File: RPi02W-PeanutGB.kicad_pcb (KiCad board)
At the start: 4 copper layers, 100 x 100 mm, 62 parts, among them J1 Raspberry_Pi_2_3, J3 AudioJack3_SwitchTR, J4 Conn_01x50, J5 Conn_02x10_Odd_Even, J6 Conn_02x10_Odd_Even, J7 Conn_02x10_Odd_Even, J8 Conn_02x10_Odd_Even, J9 USB_C_Receptacle, SW1 SW_SPDT_MSM, SW10 SW_Push, SW11 SW_Push, SW12 SW_Push, SW13 SW_Push, SW14 SW_Push, SW2 SW_Push, SW3 SW_Push, SW4 SW_Push, SW5 SW_Push, SW6 SW_Push, SW7 SW_Push, SW8 SW_Push, SW9 SW_Push, U1 MCP73831-2-OT, U3 LM4861MX

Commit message: Add files via upload
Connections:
- J1 pad 10: EXT-RXD -> unconnected-(J1-GPIO15/RXD-Pad10)
- J1 pad 3: EXT-SDA -> unconnected-(J1-SDA/GPIO2-Pad3)
- J1 pad 5: EXT-SCL -> unconnected-(J1-SCL/GPIO3-Pad5)
- J1 pad 8: EXT-TXD -> unconnected-(J1-GPIO14/TXD-Pad8)
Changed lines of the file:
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@@
   (net 12 "Net-(D1-K)")
   (net 13 "POWER")
-  (net 14 "EXT-SDA")
-  (net 15 "EXT-SCL")
+  (net 14 "unconnected-(J1-SDA{slash}GPIO2-Pad3)")
+  (net 15 "unconnected-(J1-SCL{slash}GPIO3-Pad5)")
   (net 16 "BUTTON-DU")
-  (net 17 "EXT-TXD")
-  (net 18 "EXT-RXD")
+  (net 17 "unconnected-(J1-GPIO14{slash}TXD-Pad8)")
+  (net 18 "unconnected-(J1-GPIO15{slash}RXD-Pad10)")
   (net 19 "BUTTON-START")
   (net 20 "BUTTON-RB")
@@
       (net 13 "POWER") (pinfunction "5V") (pintype "power_in"))
     (pad "3" thru_hole oval (at 0 -2.54 270) (size 1.7 1.7) (drill 1) (layers "*.Cu" "*.Mask")
-      (net 14 "EXT-SDA") (pinfunction "SDA/GPIO2") (pintype "bidirectional"))
+      (net 14 "unconnected-(J1-SDA{slash}GPIO2-Pad3)") (pinfunction "SDA/GPIO2") (pintype "bidirectional+no_connect"))
     (pad "4" thru_hole oval (at 2.54 -2.54 270) (size 1.7 1.7) (drill 1) (layers "*.Cu" "*.Mask")
       (net 13 "POWER") (pinfunction "5V") (pintype "passive"))
     (pad "5" thru_hole oval (at 0 -5.08 270) (size 1.7 1.7) (drill 1) (layers "*.Cu" "*.Mask")
-      (net 15 "EXT-SCL") (pinfunction "SCL/GPIO3") (pintype "bidirectional"))
+      (net 15 "unconnected-(J1-SCL{slash}GPIO3-Pad5)") (pinfunction "SCL/GPIO3") (pintype "bidirectional+no_connect"))
     (pad "6" thru_hole oval (at 2.54 -5.08 270) (size 1.7 1.7) (drill 1) (layers "*.Cu" "*.Mask")
       (net 2 "GND") (pinfunction "GND") (pintype "power_in"))
@@
       (net 16 "BUTTON-DU") (pinfunction "GCLK0/GPIO4") (pintype "bidirectional"))
     (pad "8" thru_hole oval (at 2.54 -7.62 270) (size 1.7 1.7) (drill 1) (layers "*.Cu" "*.Mask")
-      (net 17 "EXT-TXD") (pinfunction "GPIO14/TXD") (pintype "bidirectional"))
+      (net 17 "unconnected-(J1-GPIO14{slash}TXD-Pad8)") (pinfunction "GPIO14/TXD") (pintype "bidirectional+no_connect"))
     (pad "9" thru_hole oval (at 0 -10.16 270) (size 1.7 1.7) (drill 1) (layers "*.Cu" "*.Mask")
       (net 2 "GND") (pinfunction "GND") (pintype "passive"))
     (pad "10" thru_hole oval (at 2.54 -10.16 270) (size 1.7 1.7) (drill 1) (layers "*.Cu" "*.Mask")
-      (net 18 "EXT-RXD") (pinfunction "GPIO15/RXD") (pintype "bidirectional"))
+      (net 18 "unconnected-(J1-GPIO15{slash}RXD-Pad10)") (pinfunction "GPIO15/RXD") (pintype "bidirectional+no_connect"))
     (pad "11" thru_hole oval (at 0 -12.7 270) (size 1.7 1.7) (drill 1) (layers "*.Cu" "*.Mask")
       (net 19 "BUTTON-START") (pinfunction "GPIO17") (pintype "bidirectional"))

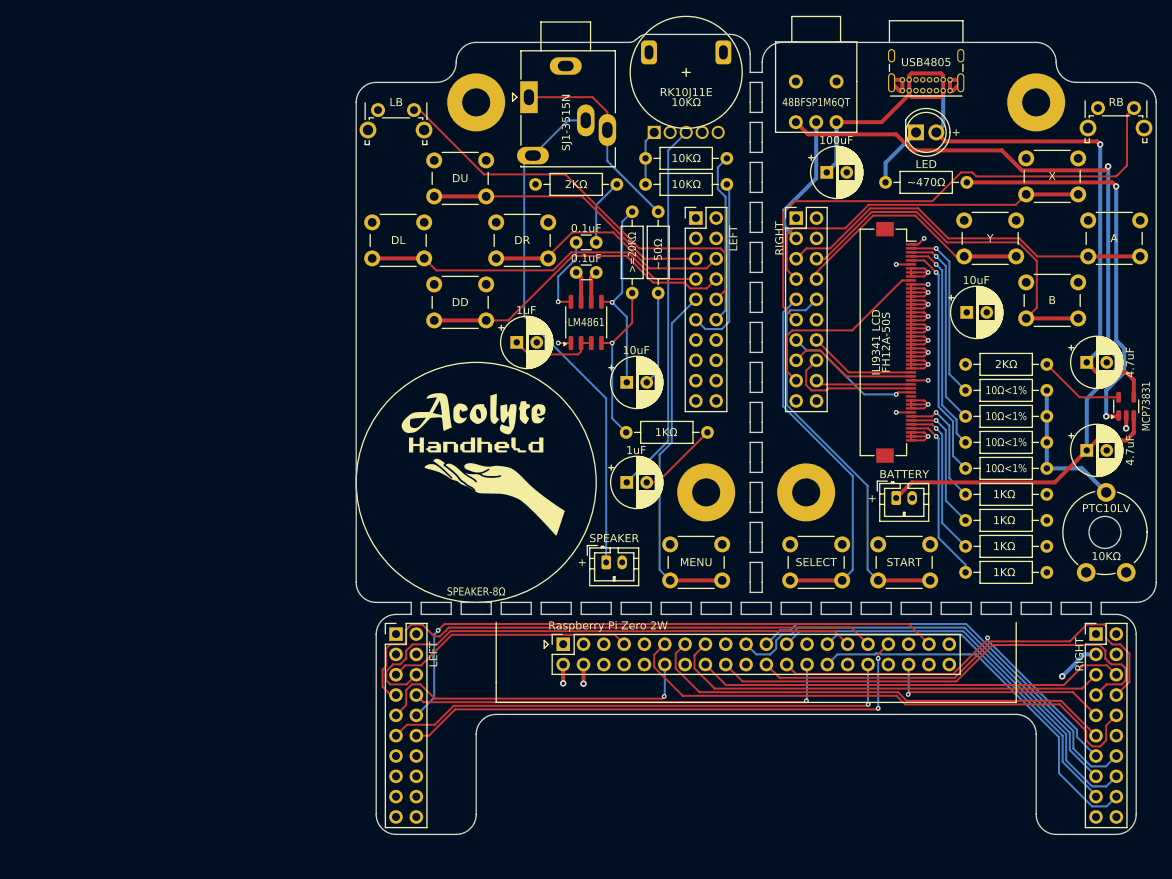
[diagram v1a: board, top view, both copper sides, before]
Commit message: Add files via upload
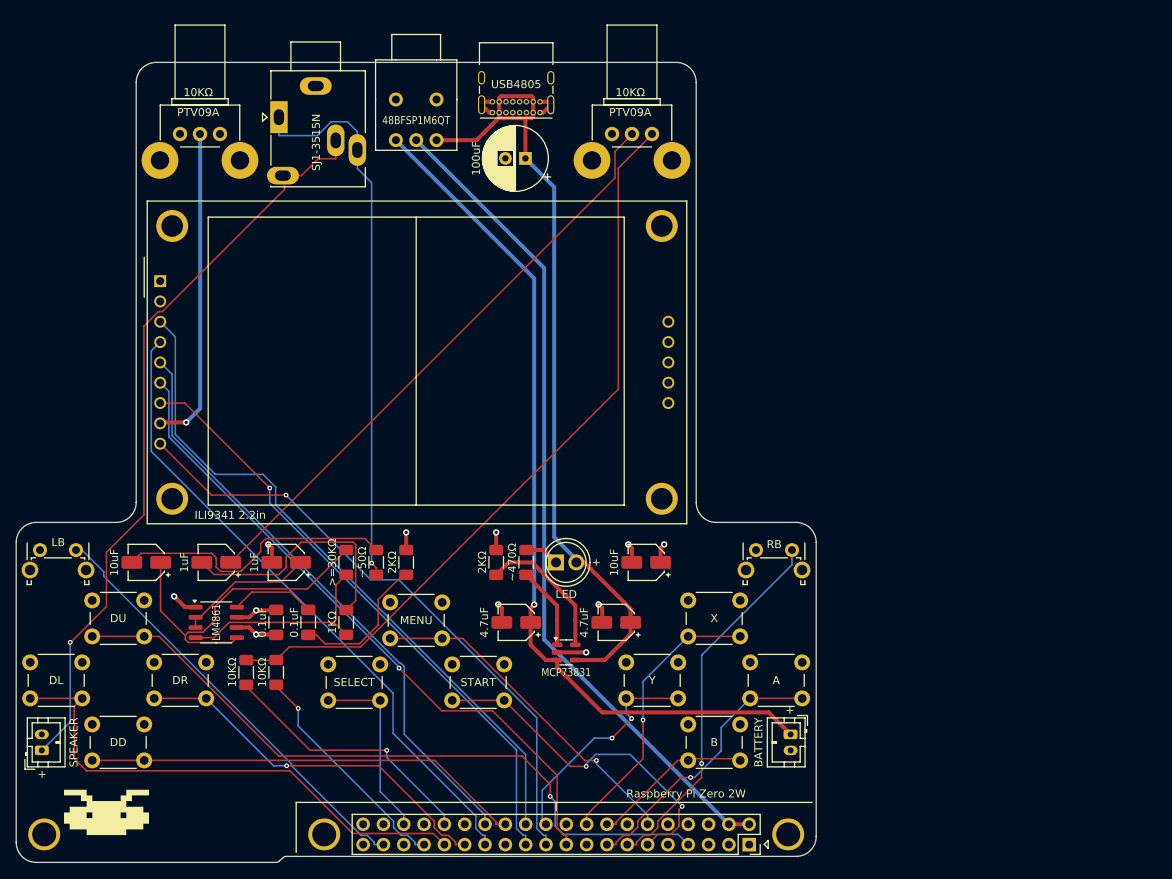
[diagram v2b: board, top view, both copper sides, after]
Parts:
- removed J4: Conn_01x50, Connector_FFC-FPC:Hirose_FH12-50S-0.5SH_1x50-1MP_P0.50mm_Horizontal
- removed J5, J6, J7, J8: Conn_02x10_Odd_Even, Connector_PinHeader_2.54mm:PinHeader_2x10_P2.54mm_Vertical
- removed R10, R11, R12, R13, R14, R15, R16, R9: R_US, Resistor_THT:R_Axial_DIN0207_L6.3mm_D2.5mm_P10.16mm_Horizontal
- removed RV1: R_Potentiometer_US, Potentiometer_THT:Potentiometer_Piher_PT-10-V10_Vertical_Hole
- removed TP4: TestPoint, RPi02W-PeanutGB:ScrewHole-4-40
- added G109: LOGO, RPi02W-PeanutGB:Alien, F.Cu at (61.2, 143.8)
- added RV3: R_Potentiometer_US, Potentiometer_THT:Potentiometer_Bourns_PTV09A-2_Single_Horizontal, F.Cu at (75.5, 59.0)
- added U4: CR2013-MI2120, Display:CR2013-MI2120, F.Cu at (68.0, 77.3)
- C1, C2, C3, C4, C5, C9: footprint Capacitor_THT:CP_Radial_D6.3mm_P2.50mm -> Capacitor_SMD:CP_Elec_4x5.8
- C6, C7: footprint Capacitor_THT:C_Disc_D3.0mm_W1.6mm_P2.50mm -> Capacitor_SMD:C_1206_3216Metric_Pad1.33x1.80mm_HandSolder
- C8: footprint Capacitor_THT:CP_Radial_D6.3mm_P2.50mm -> Capacitor_THT:CP_Radial_D8.0mm_P2.50mm
- G101, G102, G103: moved to B.Cu
- R1, R2, R3, R4, R5, R6, R7, R8: footprint Resistor_THT:R_Axial_DIN0207_L6.3mm_D2.5mm_P10.16mm_Horizontal -> Resistor_SMD:R_1206_3216Metric_Pad1.30x1.75mm_HandSolder
- RV2: footprint RPi02W-PeanutGB:RK10J1xE -> Potentiometer_THT:Potentiometer_Bourns_PTV09A-2_Single_Horizontal
- TP1, TP2, TP3: footprint RPi02W-PeanutGB:ScrewHole-4-40 -> RPi02W-PeanutGB:ScrewHole-RPiZero
- moved TP2 96.6 mm to (146.5, 146.5)
- moved TP1 93.5 mm to (88.5, 146.5)
- moved TP3 93.1 mm to (53.5, 146.5)
- moved R3 85.6 mm to (78.8, 126.2), turned to 90 degrees
- moved R4 79.1 mm to (82.5, 126.2), turned to -90 degrees
- moved U1 76.5 mm to (118.8, 123.8), turned to 0 degrees
- moved C2 74.5 mm to (112.5, 120.0), turned to 180 degrees
- moved LS1 74.4 mm to (53.2, 136.0), turned to 90 degrees
- moved R1 73.1 mm to (110.0, 112.5), turned to 90 degrees
- moved D1 70.1 mm to (117.5, 112.5)
- moved SW11 69.9 mm to (142.5, 111.0)
- moved SW2 69.7 mm to (59.5, 117.2)
- moved SW3 69.7 mm to (67.2, 125.0)
- moved SW4 69.7 mm to (51.8, 125.0)
- moved SW5 69.7 mm to (59.5, 132.8)
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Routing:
- net Net-(R3-Pad2): track 6.95 -> 94.2 mm
- net BUTTON-RB: track 127.0 -> 46.5 mm, vias 0 -> 1
- net BUTTON-B: track 100.6 -> 20.3 mm
- net POWER: track 26.9 -> 104.2 mm, vias 3 -> 0
- net BUTTON-START: track 117.7 -> 43.4 mm, vias 0 -> 2
- net BUTTON-LB: track 127.1 -> 54.3 mm, vias 1 -> 0
- net BUTTON-X: track 105.1 -> 35.2 mm, vias 0 -> 1
- net BUTTON-A: track 103.6 -> 34.3 mm, vias 0 -> 1
- net AUDIO-RIGHT: track 89.2 -> 28.8 mm, vias 2 -> 1
- net GND: track 92.7 -> 32.9 mm, vias 15 -> 9
- net BUTTON-Y: track 87.9 -> 28.6 mm, vias 0 -> 2
- net AUDIO-LEFT: track 88.0 -> 33.3 mm
- net BUTTON-SELECT: track 75.0 -> 23.2 mm, vias 1 -> 0
- net BUTTON-DD: track 98.0 -> 47.0 mm, vias 0 -> 1
- net BUTTON-DL: track 114.8 -> 65.2 mm
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- removed copper zone on In1.Cu, net POWER
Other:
- outline, holes or cut-outs redrawn
- board text added: "Battery 18650"
- board text added: "Battery LP503562"
- board text added: "Speaker"
- board text removed: "ILI9341-TFT-LCD"
- board text removed: "LEFT"
- board text removed: "RIGHT"
- board text removed: "SPEAKER-8Ω"
